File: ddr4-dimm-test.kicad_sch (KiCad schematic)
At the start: 137 parts

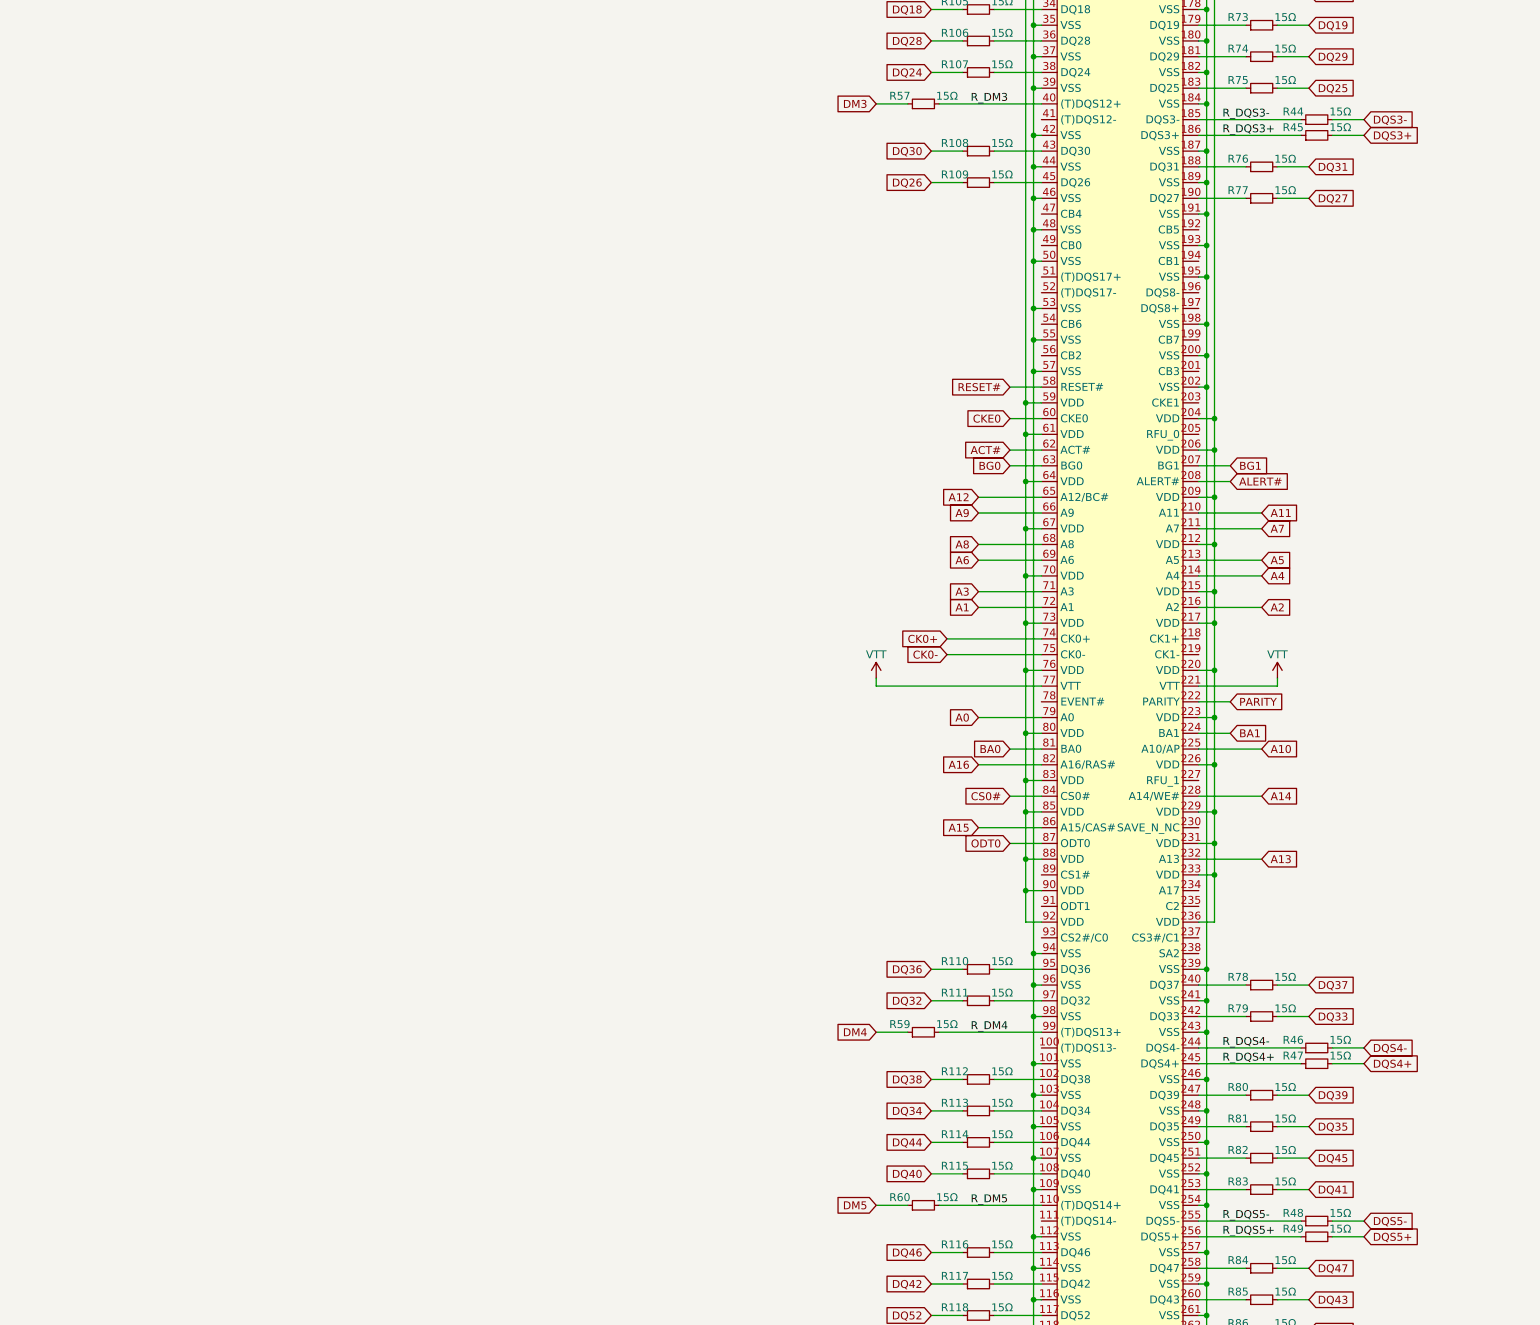
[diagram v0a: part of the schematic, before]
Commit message: Added ECC?
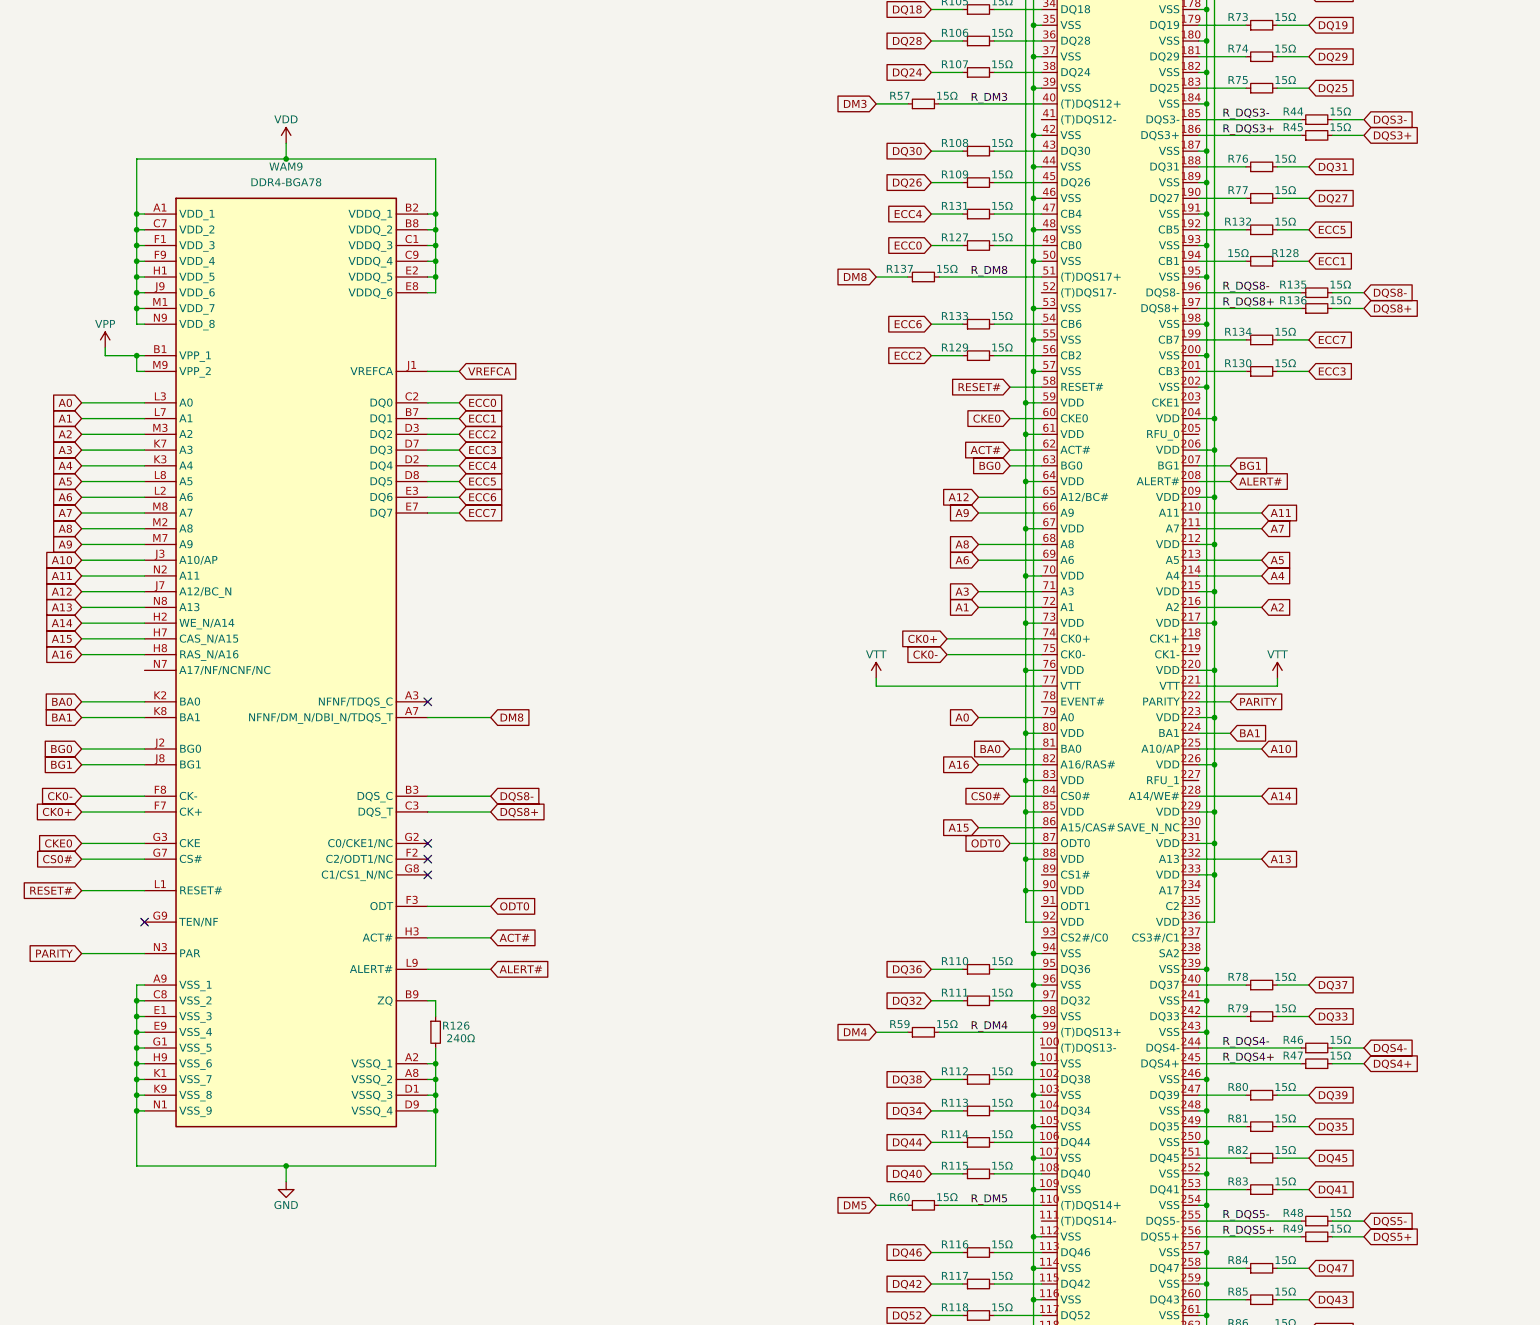
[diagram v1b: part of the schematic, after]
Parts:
- added R126: 240Ω, Resistor_SMD:R_0402_1005Metric, symbol Device:R_Small
- added R127, R128, R129, R130, R131, R132, R133, R134, R135, R136, R137: 15Ω, Resistor_SMD:R_0402_1005Metric, symbol Device:R_Small
- added WAM9: DDR4-BGA78, A_my_stuff:DDR4-BGA78, symbol A_my_stuff:DDR4-BGA78
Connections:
- net A0: now also WAM9.L3 (A0)
- net A1: now also WAM9.L7 (A1)
- net A10: now also WAM9.J3 (A10/AP)
- net A11: now also WAM9.N2 (A11)
- net A12: now also WAM9.J7 (A12/BC_N)
- net A13: now also WAM9.N8 (A13)
- net A14: now also WAM9.H2 (WE_N/A14)
- net A15: now also WAM9.H7 (CAS_N/A15)
- net A16: now also WAM9.H8 (RAS_N/A16)
- net A2: now also WAM9.M3 (A2)
- net A3: now also WAM9.K7 (A3)
- net A4: now also WAM9.K3 (A4)
- net A5: now also WAM9.L8 (A5)
- net A6: now also WAM9.L2 (A6)
- net A7: now also WAM9.M8 (A7)
- net A8: now also WAM9.M2 (A8)
- net A9: now also WAM9.M7 (A9)
- net ACT#: now also WAM9.H3 (ACT#)
- net ALERT#: now also WAM9.L9 (ALERT#)
- net BA0: now also WAM9.K2 (BA0)
- net BA1: now also WAM9.K8 (BA1)
- net BG0: now also WAM9.J2 (BG0)
- net BG1: now also WAM9.J8 (BG1)
- net CK0+: now also WAM9.F7 (CK+)
- net CK0-: now also WAM9.F8 (CK-)
- net CKE0: now also WAM9.G3 (CKE)
- net CS0#: now also WAM9.G7 (CS#)
- net GND: now also R126.2, WAM9.A2 (VSSQ_1), WAM9.A8 (VSSQ_2), WAM9.A9 (VSS_1), WAM9.C8 (VSS_2), WAM9.D1 (VSSQ_3), WAM9.D9 (VSSQ_4), WAM9.E1 (VSS_3), WAM9.E9 (VSS_4), WAM9.G1 (VSS_5), WAM9.H9 (VSS_6), WAM9.K1 (VSS_7), WAM9.K9 (VSS_8), WAM9.N1 (VSS_9)
- net ODT0: now also WAM9.F3 (ODT)
- net PARITY: now also WAM9.N3 (PAR)
- net RESET#: now also WAM9.L1 (RESET#)
- net VDD: now also WAM9.A1 (VDD_1), WAM9.B2 (VDDQ_1), WAM9.B8 (VDDQ_2), WAM9.C1 (VDDQ_3), WAM9.C7 (VDD_2), WAM9.C9 (VDDQ_4), WAM9.E2 (VDDQ_5), WAM9.E8 (VDDQ_6), WAM9.F1 (VDD_3), WAM9.F9 (VDD_4), WAM9.H1 (VDD_5), WAM9.J9 (VDD_6), WAM9.M1 (VDD_7), WAM9.N9 (VDD_8)
- net VPP: now also WAM9.B1 (VPP_1), WAM9.M9 (VPP_2)
- net VREFCA: now also WAM9.J1 (VREFCA)
- net at GF1.192 (CB5): now also R132.1
- net at GF1.194 (CB1): now also R128.2
- net R_DQS8-: now reaches GF1.196 (DQS8-)
- net R_DQS8-: now also R135.1
- net R_DQS8+: now reaches GF1.197 (DQS8+)
- net R_DQS8+: now also R136.1
- net at GF1.199 (CB7): now also R134.1
- net at GF1.201 (CB3): now also R130.1
- net at GF1.47 (CB4): now also R131.2
- net at GF1.49 (CB0): now also R127.2
- net R_DM8: now reaches GF1.51 ((T)DQS17+)
- net R_DM8: now also R137.2
- net at GF1.54 (CB6): now also R133.2
- net at GF1.56 (CB2): now also R129.2
- new net: R126.1, WAM9.B9 (ZQ)
- new net DM8: R137.1, WAM9.A7 (NFNF/DM_N/DBI_N/TDQS_T)
- new net DQS8+: R136.2, WAM9.C3 (DQS_T)
- new net DQS8-: R135.2, WAM9.B3 (DQS_C)
- new net ECC0: R127.1, WAM9.C2 (DQ0)
- new net ECC1: R128.1, WAM9.B7 (DQ1)
- new net ECC2: R129.1, WAM9.D3 (DQ2)
- new net ECC3: R130.2, WAM9.D7 (DQ3)
- new net ECC4: R131.1, WAM9.D2 (DQ4)
- new net ECC5: R132.2, WAM9.D8 (DQ5)
- new net ECC6: R133.1, WAM9.E3 (DQ6)
- new net ECC7: R134.2, WAM9.E7 (DQ7)
- no-connect marks 40 -> 45
